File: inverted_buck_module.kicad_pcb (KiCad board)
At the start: 2 copper layers, 23 x 17.5 mm, 17 parts, among them J1 Conn_01x03, U1 TPS63710

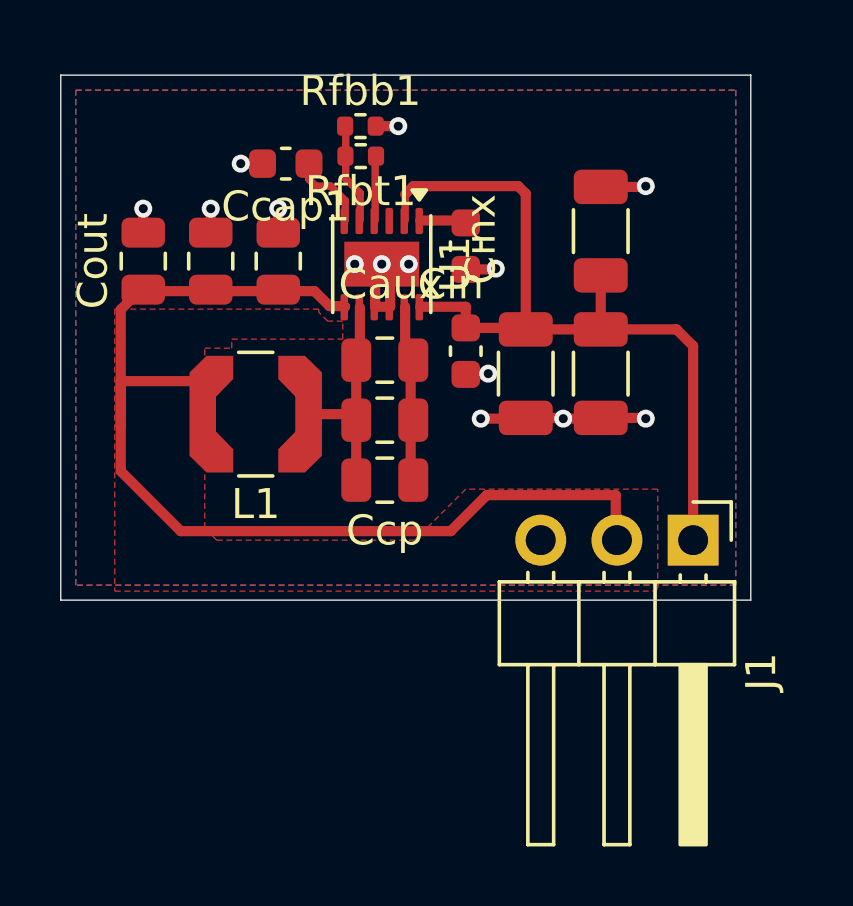
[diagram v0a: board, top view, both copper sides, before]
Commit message: fill areas
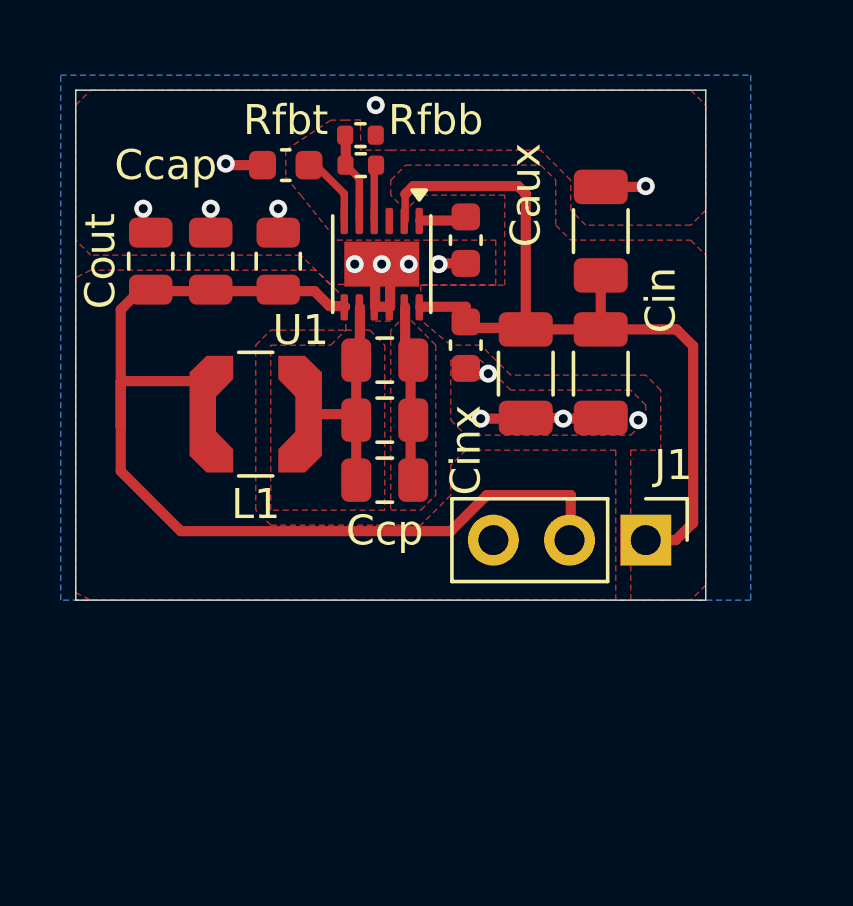
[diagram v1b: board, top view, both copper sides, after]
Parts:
- removed Ccap1: 1uF 10V, Capacitor_SMD:C_0603_1608Metric
- removed Rfbb1: 24kΩ, Resistor_SMD:R_0402_1005Metric
- removed Rfbt1: 130kΩ, Resistor_SMD:R_0402_1005Metric
- added Ccap: 1uF 10V, Capacitor_SMD:C_0603_1608Metric, F.Cu at (107.5, 52.5)
- added Rfbb: 24kΩ, Resistor_SMD:R_0402_1005Metric, F.Cu at (110.0, 51.5)
- added Rfbt: 130kΩ, Resistor_SMD:R_0402_1005Metric, F.Cu at (110.0, 52.5)
- J1: footprint Connector_PinHeader_2.54mm:PinHeader_1x03_P2.54mm_Horizontal -> Connector_PinHeader_2.54mm:PinHeader_1x03_P2.54mm_Vertical
- moved J1 1.58 mm to (119.5, 65.0)
- moved Cout 0.25 mm to (103.0, 55.7)
- moved Caux 0.20 mm to (113.5, 55.0)
- moved Cinx 0.20 mm to (113.5, 58.5)
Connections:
- net Net-(U1-CP) renamed /CP
- net Net-(U1-SW) renamed /SW
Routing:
- net GND: track 16.3 -> 14.1 mm
- net Vin: track 27.2 -> 29.2 mm
- net Vout: track 36.1 -> 35.4 mm
- added copper zone on F.Cu, net /CP
- added copper zone on F.Cu, net /SW
- added copper zone on F.Cu, net Vin
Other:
- board size 23 x 17.5 mm -> 21 x 17 mm
